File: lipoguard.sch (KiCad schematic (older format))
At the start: 11 parts, among them P1 CONN_2, P2 CONN_2, Q1 BC 850C, U1 BTS6143

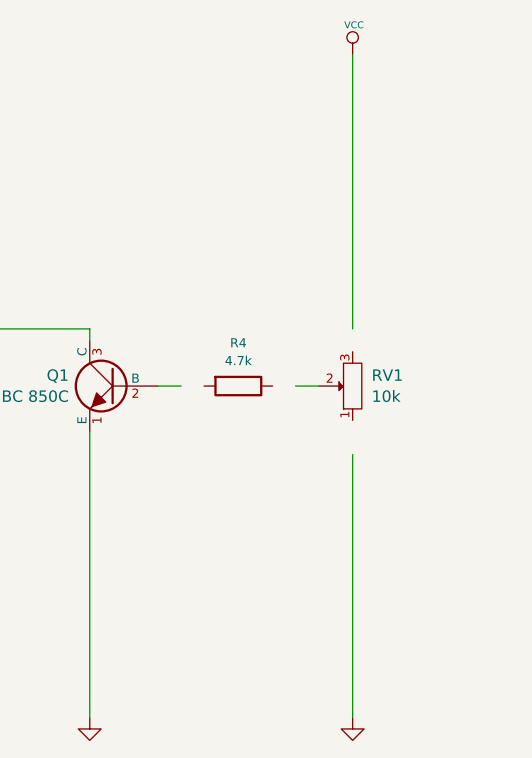
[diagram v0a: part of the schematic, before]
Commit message: Finished cleaning up
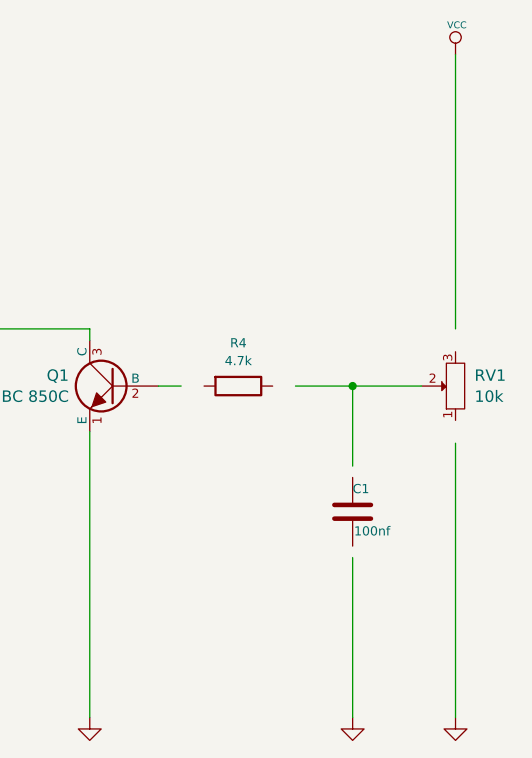
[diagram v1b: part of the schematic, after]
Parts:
- added C1: 100nf, libcms:SM0603, symbol C
- Q1: footprint (none) -> misc:sot23BEC
- R3: footprint discret:R3 -> libcms:SM0603
- R4: footprint (none) -> libcms:SM0603
- RV1: footprint (none) -> misc:trimmer1
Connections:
- wire segments 25 -> 27
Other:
- moved on the sheet: RV1
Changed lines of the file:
@@
 F 0 "R3" H 5971 4489 40  0000 L CNN
 F 1 "R" H 5971 4411 40  0000 L CNN
-F 2 "discret:R3" V 5830 4450 30  0001 C CNN
+F 2 "libcms:SM0603" V 5830 4450 30  0001 C CNN
 F 3 "" H 5900 4450 30  0000 C CNN
 	1    5900 4450
@@
 F 0 "Q1" H 6891 3946 50  0000 L CNN
 F 1 "BC 850C" H 6891 3854 50  0000 L CNN
-F 2 "" H 6700 3900 60  0000 C CNN
+F 2 "misc:sot23BEC" H 6700 3900 60  0001 C CNN
 F 3 "" H 6700 3900 60  0000 C CNN
 	1    6700 3900
@@
 F 0 "R4" V 7062 3900 40  0000 C CNN
 F 1 "4.7k" V 7140 3900 40  0000 C CNN
-F 2 "" V 7180 3900 30  0000 C CNN
+F 2 "libcms:SM0603" V 7180 3900 30  0001 C CNN
 F 3 "" H 7250 3900 30  0000 C CNN
 	1    7250 3900
@@
 L POT RV1
 U 1 1 57F26A5C
-P 7750 3900
-F 0 "RV1" V 7796 3817 50  0000 R CNN
-F 1 "10k" V 7704 3817 50  0000 R CNN
-F 2 "" H 7750 3900 60  0000 C CNN
-F 3 "" H 7750 3900 60  0000 C CNN
-	1    7750 3900
+P 8200 3900
+F 0 "RV1" V 8246 3817 50  0000 R CNN
+F 1 "10k" V 8154 3817 50  0000 R CNN
+F 2 "misc:trimmer1" H 8200 3900 60  0001 C CNN
+F 3 "" H 8200 3900 60  0000 C CNN
+	1    8200 3900
 	0    -1   -1   0
 $EndComp
 Wire Wire Line
-	7500 3900 7600 3900
-Wire Wire Line
-	7750 4200 7750 5350
+	7500 3900 8050 3900
+Wire Wire Line
+	8200 4150 8200 5350
 $Comp
 L GND #PWR010
 U 1 1 57F26B56
-P 7750 5350
-F 0 "#PWR010" H 7750 5350 30  0001 C CNN
-F 1 "GND" H 7750 5280 30  0001 C CNN
-F 2 "" H 7750 5350 60  0000 C CNN
-F 3 "" H 7750 5350 60  0000 C CNN
-	1    7750 5350
-	1    0    0    -1
-$EndComp
-Wire Wire Line
-	7750 3650 7750 2450
+P 8200 5350
+F 0 "#PWR010" H 8200 5350 30  0001 C CNN
+F 1 "GND" H 8200 5280 30  0001 C CNN
+F 2 "" H 8200 5350 60  0000 C CNN
+F 3 "" H 8200 5350 60  0000 C CNN
+	1    8200 5350
+	1    0    0    -1
+$EndComp
+Wire Wire Line
+	8200 3650 8200 2450
 $Comp
 L VCC #PWR011
 U 1 1 57F26BA7
-P 7750 2450
-F 0 "#PWR011" H 7750 2550 30  0001 C CNN
-F 1 "VCC" H 7756 2579 30  0000 C CNN
-F 2 "" H 7750 2450 60  0000 C CNN
-F 3 "" H 7750 2450 60  0000 C CNN
-	1    7750 2450
-	1    0    0    -1
-$EndComp
+P 8200 2450
+F 0 "#PWR011" H 8200 2550 30  0001 C CNN
+F 1 "VCC" H 8206 2579 30  0000 C CNN
+F 2 "" H 8200 2450 60  0000 C CNN
+F 3 "" H 8200 2450 60  0000 C CNN
+	1    8200 2450
+	1    0    0    -1
+$EndComp
+$Comp
+L C C1
+U 1 1 57F3D205
+P 7750 4450
+F 0 "C1" H 7750 4550 40  0000 L CNN
+F 1 "100nf" H 7756 4365 40  0000 L CNN
+F 2 "libcms:SM0603" H 7788 4300 30  0001 C CNN
+F 3 "" H 7750 4450 60  0000 C CNN
+	1    7750 4450
+	1    0    0    -1
+$EndComp
+Wire Wire Line
+	7750 4250 7750 3900
+Connection ~ 7750 3900
+Wire Wire Line
+	7750 4650 7750 5350
+$Comp
+L GND #PWR012
+U 1 1 57F3D38A
+P 7750 5350
+F 0 "#PWR012" H 7750 5350 30  0001 C CNN
+F 1 "GND" H 7750 5280 30  0001 C CNN
+F 2 "" H 7750 5350 60  0001 C CNN
+F 3 "" H 7750 5350 60  0001 C CNN
+	1    7750 5350
+	1    0    0    -1
+$EndComp
